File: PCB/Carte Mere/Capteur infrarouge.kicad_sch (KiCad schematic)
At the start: 15 parts, among them J10 TRCT5000, J11 TRCT5000, J5 IR204, J6 IR204, J7 TL1838, J8 TRCT5000, J9 TRCT5000

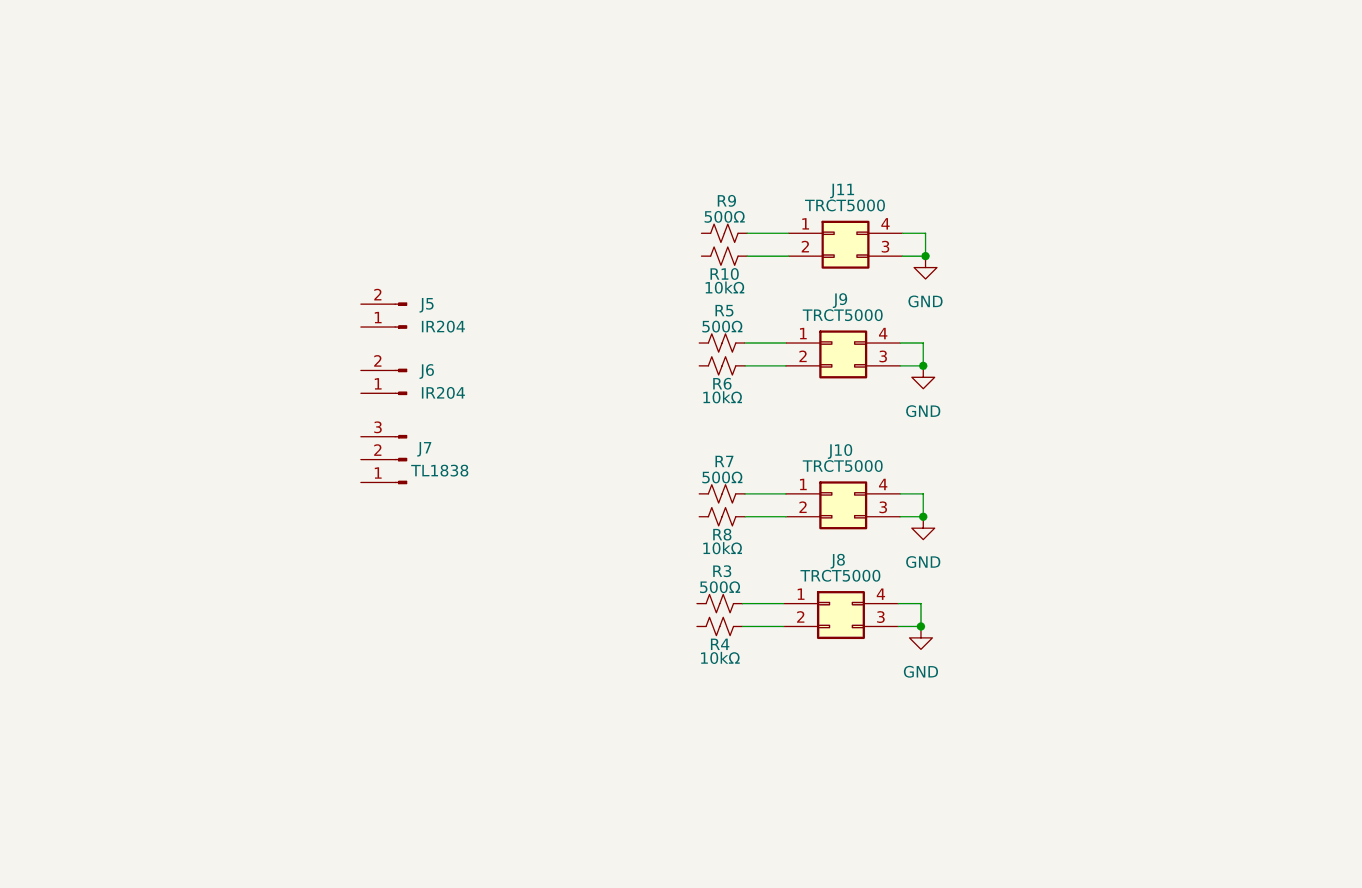
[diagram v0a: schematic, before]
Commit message: 1.5 PCB
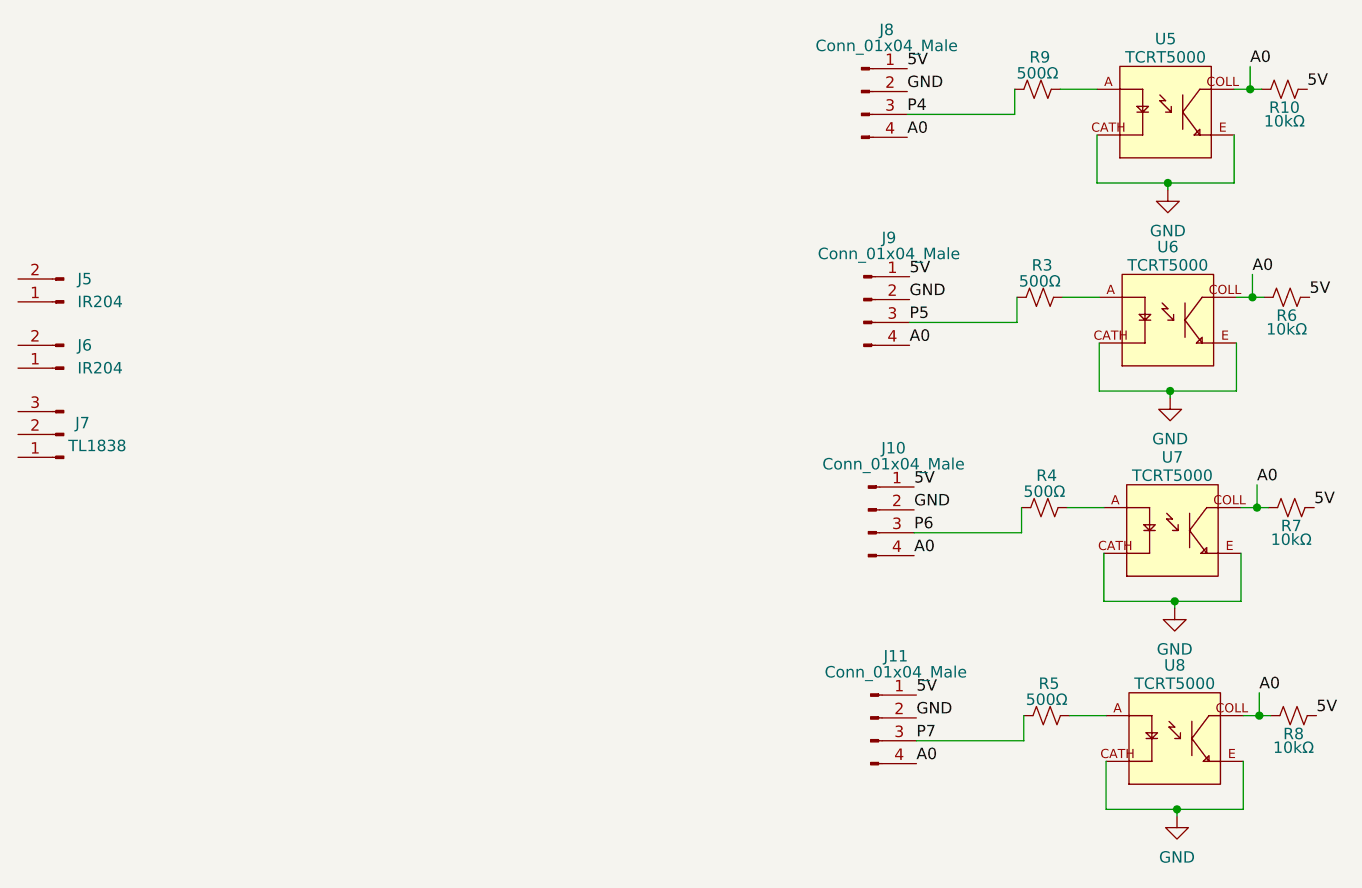
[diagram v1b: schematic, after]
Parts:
- removed J10, J11, J8, J9: TRCT5000, symbol Connector_Generic:Conn_02x02_Counter_Clockwise
- added J10, J11, J8, J9: Conn_01x04_Male, symbol Connector:Conn_01x04_Male
- added U5, U6, U7, U8: TCRT5000, symbol TCRT5000:TCRT5000
- R4: value 10kΩ -> 500Ω
- R7: value 500Ω -> 10kΩ
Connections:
- net GND: now also J10.2 (Pin_2), J11.2 (Pin_2), J8.2 (Pin_2), J9.2 (Pin_2), U5.CATH, U5.E, U6.CATH, U6.E, U7.CATH, U7.E, U8.CATH, U8.E
- net at R3.2: now also U6.A
- net at R4.2: now also U7.A
- net A0: now reaches R10.1
- net A0: now also R6.1, R7.1, R8.1, J10.4 (Pin_4), J11.4 (Pin_4), J8.4 (Pin_4), J9.4 (Pin_4), U5.COLL, U6.COLL, U7.COLL, U8.COLL
- net 5V: now reaches R10.2
- net 5V: now also R6.2, R7.2, R8.2, J10.1 (Pin_1), J11.1 (Pin_1), J8.1 (Pin_1), J9.1 (Pin_1)
- net P6: now reaches R4.1
- net P6: now also J10.3 (Pin_3)
- net P5: now reaches R3.1
- net P5: now also J9.3 (Pin_3)
- net at R5.2: now also U8.A
- net P4: now reaches R9.1
- net P4: now also J8.3 (Pin_3)
- net at R9.2: now also U5.A
- net P7: now reaches R5.1
- net P7: now also J11.3 (Pin_3)
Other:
- moved on the sheet: J5, J6, J7, R10, R9
